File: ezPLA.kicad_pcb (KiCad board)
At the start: 2 copper layers, 24.5 x 40 mm, 5 parts, among them J1 JTAG-10, J2 Power, J3 PLA-headers, U2 EPM7032

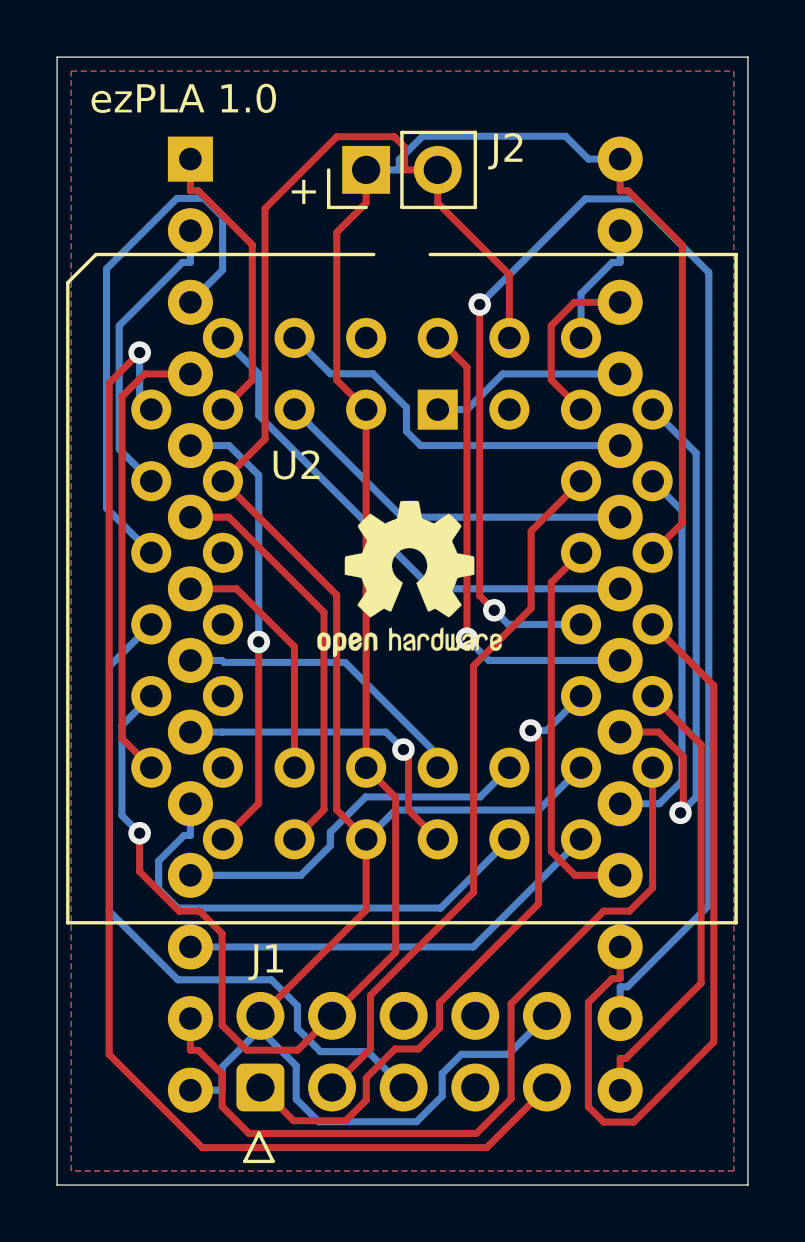
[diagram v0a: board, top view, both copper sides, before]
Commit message: Update KiCad files
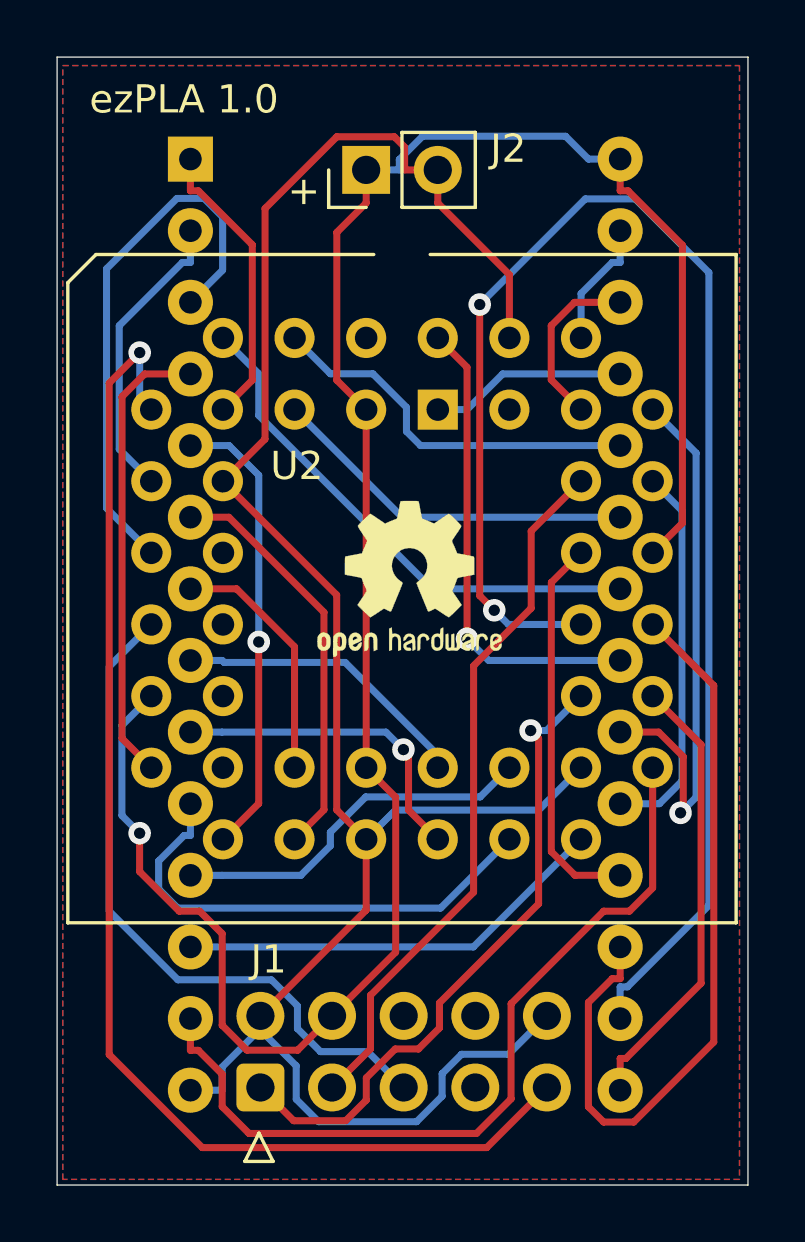
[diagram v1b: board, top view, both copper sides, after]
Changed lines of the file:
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@@
-(kicad_pcb (version 20171130) (host pcbnew "(5.1.8-0-10_14)")
+(kicad_pcb (version 20171130) (host pcbnew "(5.1.10)-1")
   (general
     (thickness 1.6)
@@
     (pad_to_mask_clearance 0)
     (aux_axis_origin 0 0)
-    (visible_elements FFFFFF7F)
+    (visible_elements 7FFFFFFF)
     (pcbplotparams
       (layerselection 0x010fc_ffffffff)
@@
       (effects (font (size 1 1) (thickness 0.15)))
     )
-    (fp_text user %R (at 1.27 5.08 180) (layer F.Fab)
-      (effects (font (size 1 1) (thickness 0.15)))
-    )
     (fp_line (start -2.6226 0.4492) (end -1.6226 -0.0508) (layer F.SilkS) (width 0.12))
     (fp_line (start -2.6226 -0.5508) (end -2.6226 0.4492) (layer F.SilkS) (width 0.12))
     (fp_line (start -1.6226 -0.0508) (end -2.6226 -0.5508) (layer F.SilkS) (width 0.12))
+    (fp_text user %R (at 1.27 5.08 180) (layer F.Fab)
+      (effects (font (size 1 1) (thickness 0.15)))
+    )
     (pad 1 thru_hole roundrect (at 0 0 90) (size 1.7 1.7) (drill 1) (layers *.Cu *.Mask) (roundrect_rratio 0.1470588235294118)
       (net 15 TCK))
@@
       (effects (font (size 1 1) (thickness 0.15)) (justify mirror))
     )
-    (fp_text user %R (at 0.1524 -0.127) (layer B.Fab)
-      (effects (font (size 1 1) (thickness 0.15)) (justify mirror))
-    )
-    (fp_arc (start 0.1524 17.713) (end 1.1524 17.713) (angle -180) (layer B.SilkS) (width 0.12))
     (fp_line (start -8.5276 17.933) (end 8.8224 17.933) (layer B.CrtYd) (width 0.05))
     (fp_line (start -8.5276 -18.167) (end -8.5276 17.933) (layer B.CrtYd) (width 0.05))
@@
     (fp_line (start -7.2126 17.653) (end -7.2126 -17.907) (layer B.Fab) (width 0.1))
     (fp_line (start 6.5174 17.653) (end -7.2126 17.653) (layer B.Fab) (width 0.1))
+    (fp_text user %R (at 0.1524 -0.127) (layer B.Fab)
+      (effects (font (size 1 1) (thickness 0.15)) (justify mirror))
+    )
+    (fp_arc (start 0.1524 17.713) (end 1.1524 17.713) (angle -180) (layer B.SilkS) (width 0.12))
     (pad 28 thru_hole oval (at -7.4676 16.383 180) (size 1.6 1.6) (drill 0.8) (layers *.Cu *.Mask)
       (net 11 VCC))
@@
       (effects (font (size 1 1) (thickness 0.15)))
     )
-    (fp_text user %R (at 0 1.27) (layer F.Fab)
-      (effects (font (size 1 1) (thickness 0.15)))
-    )
     (fp_line (start -0.635 -1.27) (end 1.27 -1.27) (layer F.Fab) (width 0.1))
     (fp_line (start 1.27 -1.27) (end 1.27 3.81) (layer F.Fab) (width 0.1))
@@
     (fp_line (start 1.8 4.35) (end 1.8 -1.8) (layer F.CrtYd) (width 0.05))
     (fp_line (start 1.8 -1.8) (end -1.8 -1.8) (layer F.CrtYd) (width 0.05))
+    (fp_text user %R (at 0 1.27) (layer F.Fab)
+      (effects (font (size 1 1) (thickness 0.15)))
+    )
     (pad 2 thru_hole oval (at 0 2.54 90) (size 1.7 1.7) (drill 1) (layers *.Cu *.Mask)
       (net 10 GND))
@@
     )
     (fp_text value EPM7032 (at -1 8) (layer F.Fab)
-      (effects (font (size 1 1) (thickness 0.15)))
-    )
-    (fp_text user %R (at -1.27 6.35) (layer F.Fab)
       (effects (font (size 1 1) (thickness 0.15)))
     )
@@
     (fp_line (start 10.58 18.2) (end 10.58 -5.5) (layer F.SilkS) (width 0.12))
     (fp_line (start 10.58 -5.5) (end -0.27 -5.5) (layer F.SilkS) (width 0.12))
+    (fp_text user %R (at -1.27 6.35) (layer F.Fab)
+      (effects (font (size 1 1) (thickness 0.15)))
+    )
     (pad 39 thru_hole circle (at 7.62 0) (size 1.4224 1.4224) (drill 0.8) (layers *.Cu *.Mask)
       (net 30 VA12))
@@
     (polygon
       (pts
-        (xy 159.5 138.5) (xy 136 138.5) (xy 136 99.5) (xy 159.5 99.5)
+        (xy 159.7 138.8) (xy 135.7 138.8) (xy 135.7 99.3) (xy 159.7 99.3)
       )
     )
@@
     (polygon
       (pts
-        (xy 159.5 138.5) (xy 136 138.5) (xy 136 99.5) (xy 159.5 99.5)
+        (xy 159.7 138.8) (xy 135.7 138.8) (xy 135.7 99.3) (xy 159.7 99.3)
       )
     )
